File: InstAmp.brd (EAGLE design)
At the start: 38.1 x 19.1 mm, 35 parts, among them IC1 AD8221ARZ, IC2 TLC2254ID

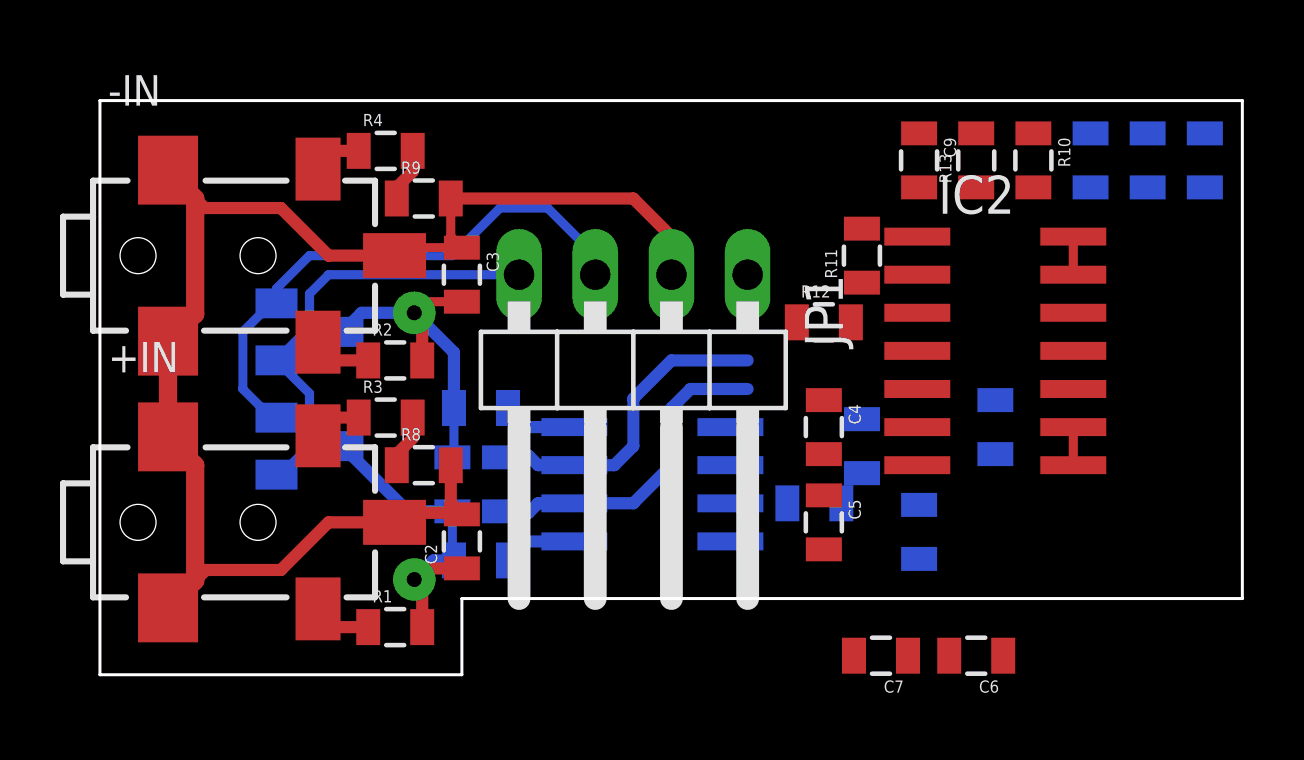
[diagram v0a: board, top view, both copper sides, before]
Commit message: .
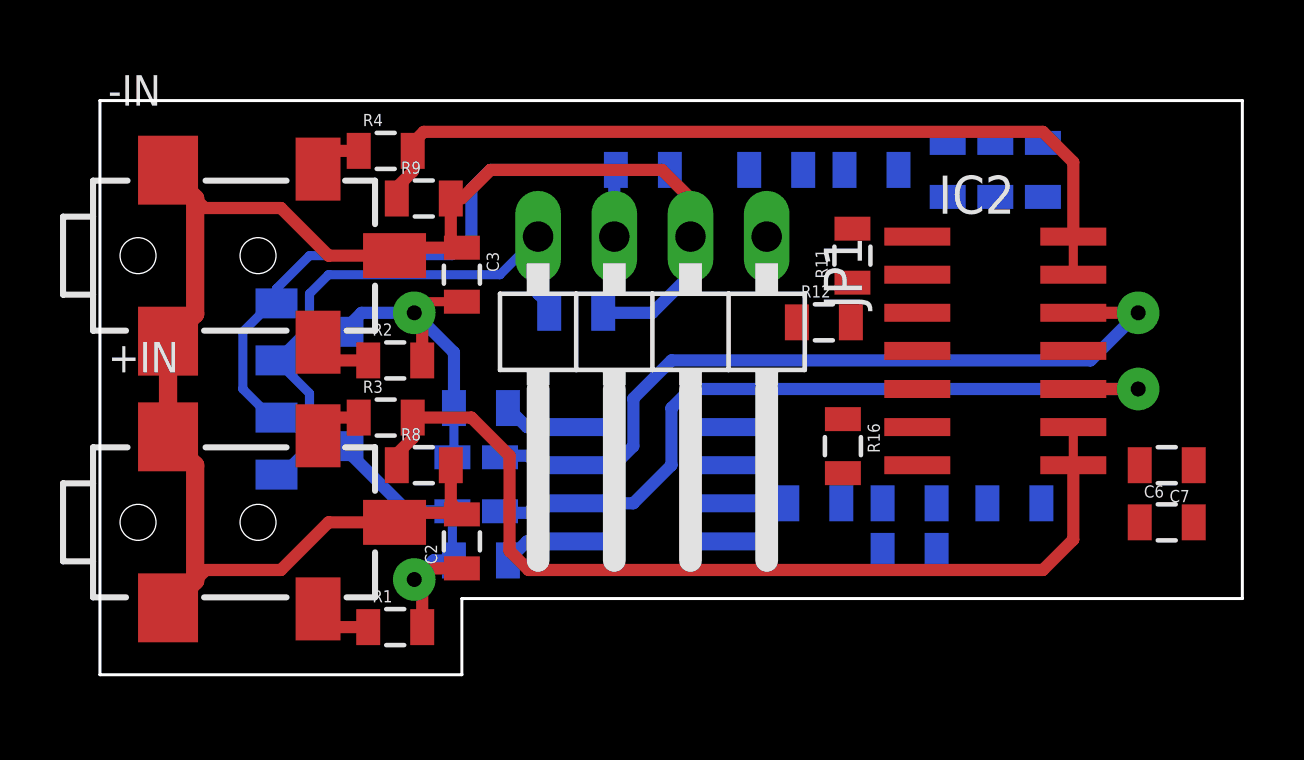
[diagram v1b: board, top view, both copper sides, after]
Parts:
- moved C5 13.2 mm to (18.1, 14.3), flipped to the bottom, turned to 0 degrees
- moved R13 11.5 mm to (30.5, 3.17), flipped to the bottom, turned to 180 degrees
- moved C7 11.4 mm to (35.6, 4.45)
- moved C4 9.09 mm to (15.9, 9.53), flipped to the bottom, turned to 180 degrees
- moved C6 7.75 mm to (35.6, 2.54), turned to 0 degrees
- moved R10 5.41 mm to (25.7, 14.3), flipped to the bottom, turned to 180 degrees
- moved R17 5.41 mm to (31.4, 14.3), turned to 90 degrees
- moved R14 5.09 mm to (29.8, 14.3), turned to 90 degrees
- moved C11 5.02 mm to (27.0, 1.59), turned to 180 degrees
- moved C8 4.77 mm to (28.3, 14.3), turned to 270 degrees
- moved C9 4.77 mm to (22.5, 14.3), flipped to the bottom, turned to 0 degrees
- moved JP1 1.42 mm to (18.4, 8.26)
- moved R15 1.00 mm to (27.0, 3.17), turned to 180 degrees
- moved R16 0.63 mm to (24.8, 5.08), flipped to the top
- moved R11 0.32 mm to (25.1, 11.4)
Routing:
- net N$17: track 3.08 -> 32.0 mm
- net N$7: track 3.08 -> 28.4 mm
- net N$8: track 10.8 -> 26.6 mm, vias 0 -> 1
- net N$16: track 11.1 -> 26.3 mm, vias 0 -> 1
- net GND: track 48.8 -> 56.9 mm
- net -5V: track 14.7 -> 18.6 mm
- net +5V: track 18.5 -> 21.6 mm

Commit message: Amp routing
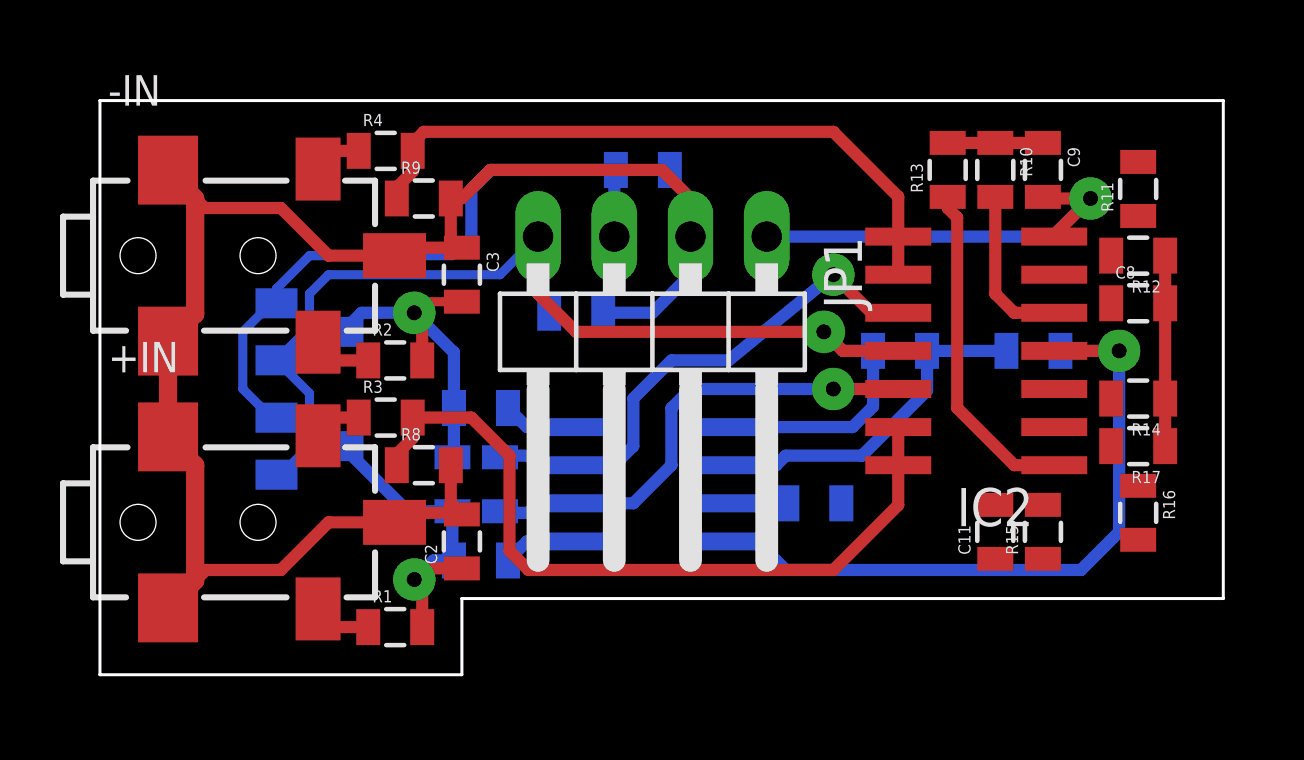
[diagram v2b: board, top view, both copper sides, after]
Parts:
- moved R13 11.3 mm to (28.3, 14.3), flipped to the top, turned to 90 degrees
- moved R12 10.7 mm to (34.6, 11.4), turned to 180 degrees
- moved R16 10.1 mm to (34.6, 2.86)
- moved R11 9.78 mm to (34.6, 13.7)
- moved R17 9.74 mm to (34.6, 5.08), flipped to the top, turned to 180 degrees
- moved C7 9.67 mm to (26.7, 8.26), flipped to the bottom, turned to 0 degrees
- moved R14 8.99 mm to (34.6, 6.67), flipped to the top, turned to 180 degrees
- moved C9 8.89 mm to (31.4, 14.3), flipped to the top, turned to 270 degrees
- moved C8 7.75 mm to (34.6, 9.84), flipped to the top, turned to 0 degrees
- moved C6 7.24 mm to (31.1, 8.26), flipped to the bottom
- moved R15 4.55 mm to (31.4, 2.22), flipped to the top, turned to 90 degrees
- moved R10 4.13 mm to (29.8, 14.3), flipped to the top, turned to 270 degrees
- moved C11 2.93 mm to (29.8, 2.22), flipped to the top, turned to 90 degrees
- moved IC2 0.63 mm to (29.2, 8.26), turned to 90 degrees
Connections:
- net N$10: now also IC2.2; no longer IC2.6
- net N$14: now also IC2.5; no longer IC2.3
- net N$16: now also IC2.12; no longer IC2.10
- net N$17: now also IC2.13, IC2.14; no longer IC2.8, IC2.9
- net N$22: now also IC2.3; no longer IC2.5
- net N$23: now also IC2.6; no longer IC2.2
- net N$7: now also IC2.8, IC2.9; no longer IC2.13, IC2.14
- net N$8: now also IC2.10; no longer IC2.12
- net N$9: now also IC2.1; no longer IC2.7
- net OUT: now also IC2.7; no longer IC2.1
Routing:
- net +5V: track 21.6 -> 45.6 mm, vias 0 -> 1
- net -5V: track 18.6 -> 42.1 mm, vias 0 -> 1
- net GND: track 56.9 -> 74.8 mm
- net OUT: track 0.00 -> 14.7 mm, vias 0 -> 1
- net N$9: track 0.00 -> 11.2 mm
- net N$16: track 26.3 -> 16.1 mm
- net N$8: track 26.6 -> 17.4 mm
- net N$7: track 28.4 -> 21.9 mm
- net N$17: track 32.0 -> 25.5 mm
- net N$14: track 0.00 -> 5.46 mm
- net N$15: track 0.00 -> 3.18 mm
- net N$11: track 0.00 -> 1.90 mm
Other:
- board size 38.1 x 19.1 mm -> 37.4 x 19.1 mm
